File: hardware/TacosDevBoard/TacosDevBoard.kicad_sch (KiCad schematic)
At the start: 11 parts, among them IC2_COMM1 Conn_01x08_Socket, J1 Conn_01x08_Socket, J2 Conn_01x08_Socket, J3 Conn_01x08_Socket, J4 Conn_01x08_Socket, J5 Conn_01x08_Socket, J7 Conn_02x17_Counter_Clockwise, J9 Conn_01x10_Pin

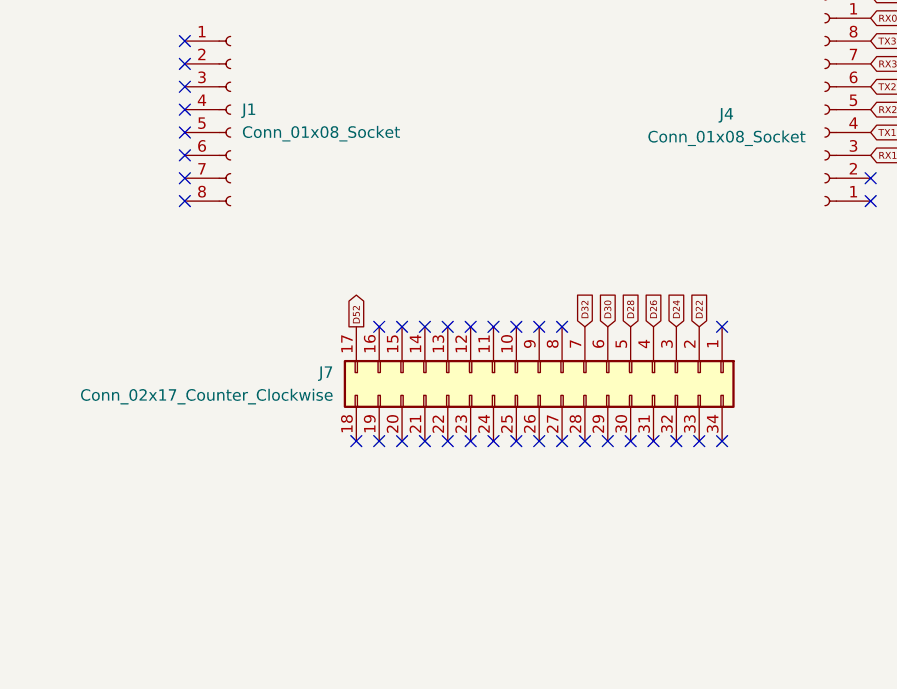
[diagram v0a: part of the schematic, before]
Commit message: started adding SD card
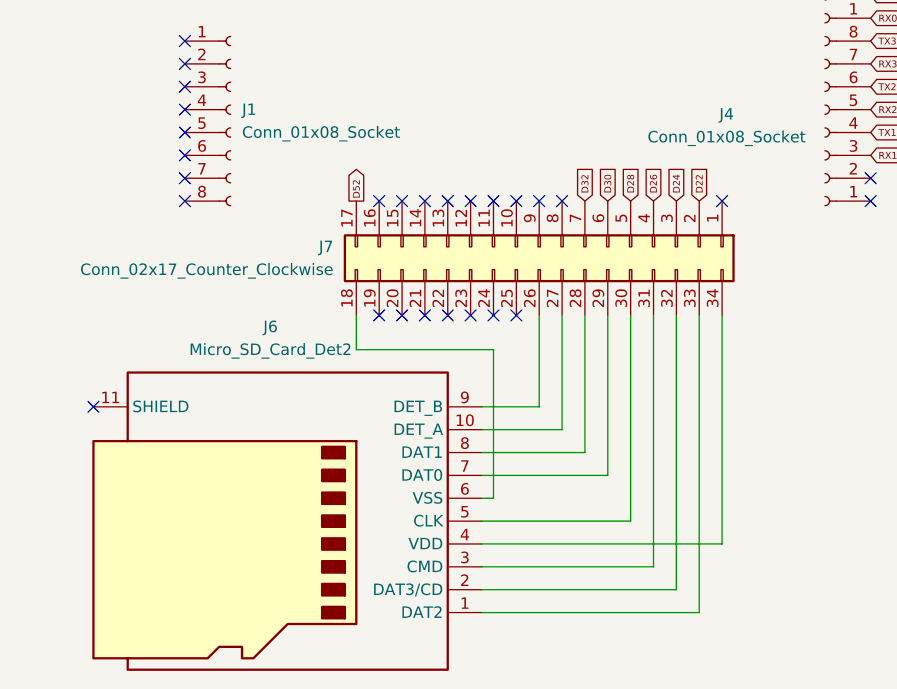
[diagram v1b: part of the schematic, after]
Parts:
- added J6: Micro_SD_Card_Det2, Connector_Card:microSD_HC_Molex_104031-0811, symbol Connector:Micro_SD_Card_Det2
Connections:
- net at J7.18 (Pin_18): now also J6.6 (VSS)
- net at J7.26 (Pin_26): now also J6.9 (DET_B)
- net at J7.27 (Pin_27): now also J6.10 (DET_A)
- net at J7.28 (Pin_28): now also J6.8 (DAT1)
- net at J7.29 (Pin_29): now also J6.7 (DAT0)
- net at J7.30 (Pin_30): now also J6.5 (CLK)
- net at J7.31 (Pin_31): now also J6.3 (CMD)
- net at J7.32 (Pin_32): now also J6.2 (DAT3/CD)
- net at J7.33 (Pin_33): now also J6.1 (DAT2)
- net at J7.34 (Pin_34): now also J6.4 (VDD)
- no-connect marks 56 -> 47
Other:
- moved on the sheet: J7
